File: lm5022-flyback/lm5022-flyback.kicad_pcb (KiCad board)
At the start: 2 copper layers, 80 x 80 mm, 55 parts, among them Q1 EPC2302, SW1 SW_Nidec_CAS-120A1, T1 Arthur, U1 LM5022MM, U2 TLVH431BQDCKT, U3 LTV-817-C

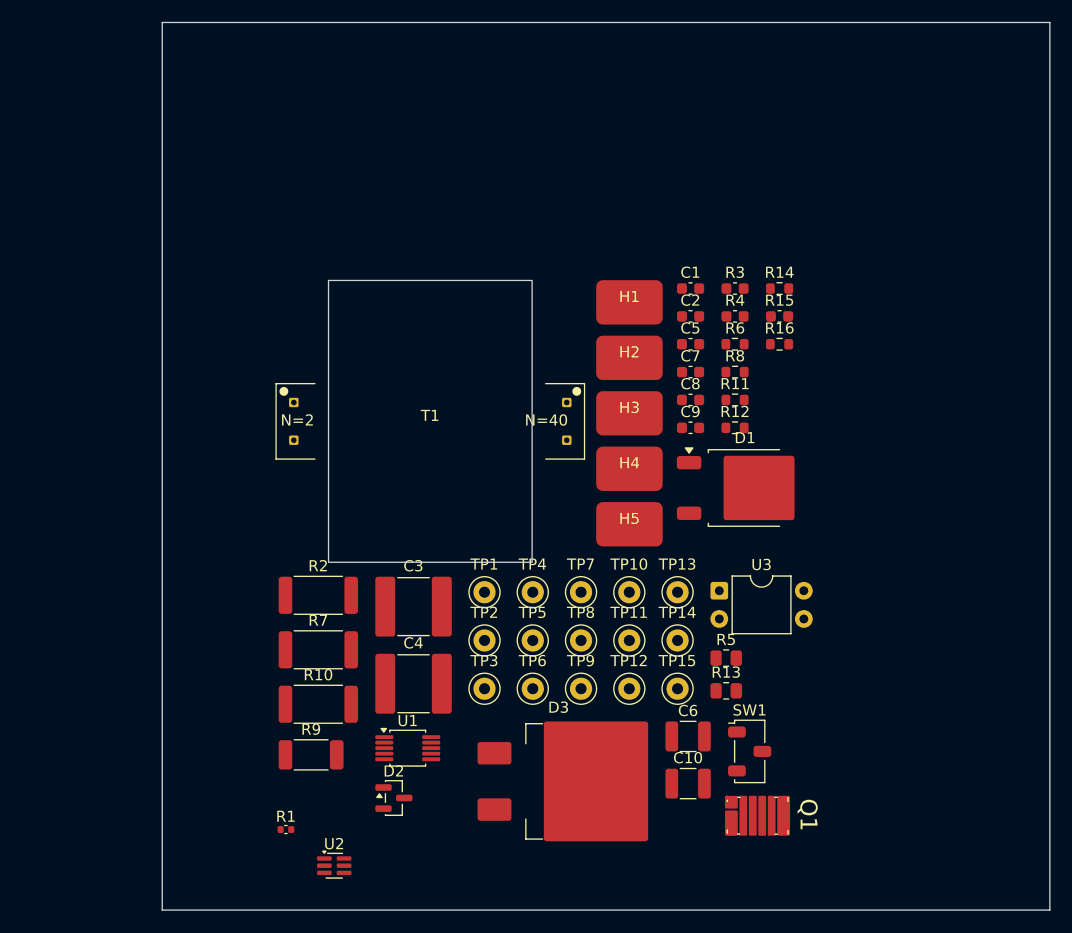
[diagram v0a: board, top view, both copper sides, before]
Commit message: layout work
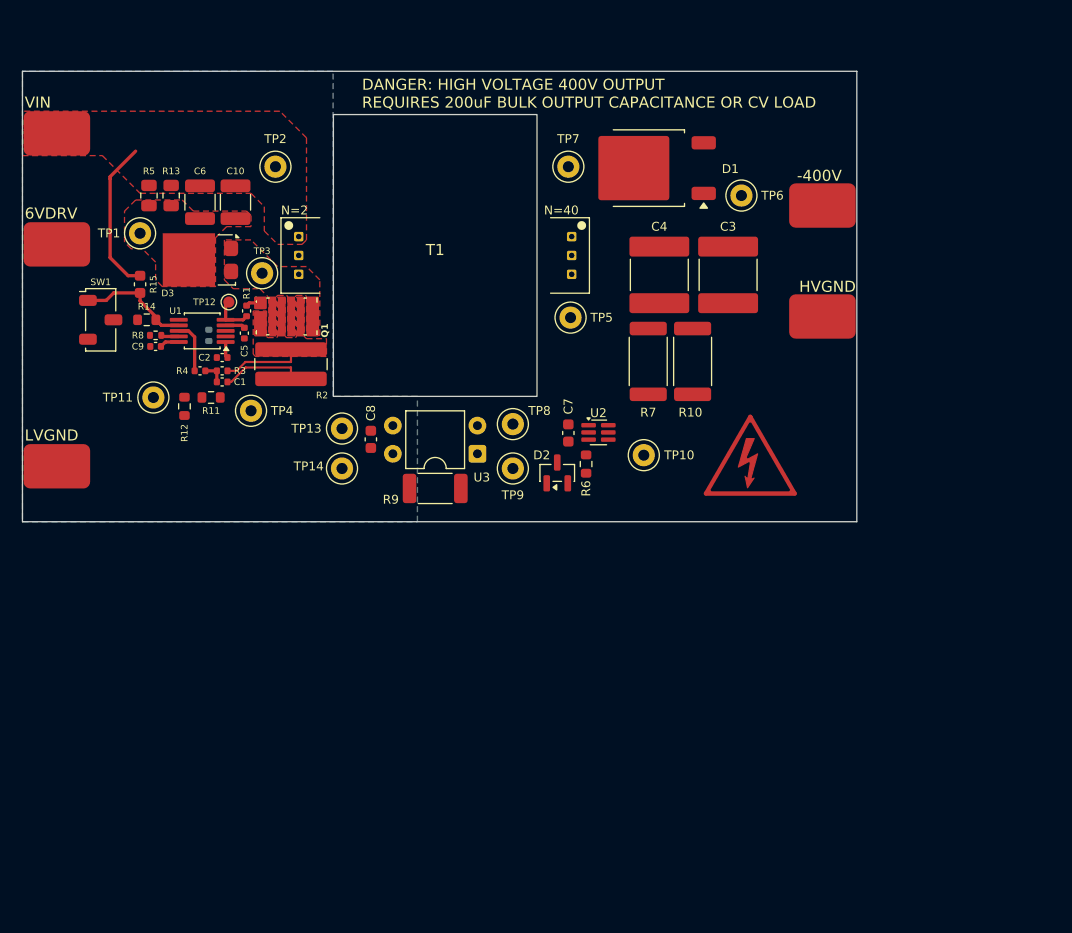
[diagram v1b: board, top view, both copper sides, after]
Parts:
- removed TP15: 5004, TestPoint:TestPoint_Keystone_5000-5004_Miniature
- added REF**: Symbol_HighVoltage_Triangle_8x7mm_Copper, Symbol:Symbol_HighVoltage_Triangle_8x7mm_Copper, F.Cu at (123.0, 104.0)
- C1, C2, C5, C9, R3, R4: footprint Capacitor_SMD:C_0603_1608Metric -> Capacitor_SMD:C_0402_1005Metric
- C8: value 100pF DNP -> 100pF
- D3: value V40D103C-M3/I -> PPH10100; footprint TO_SOT_SMD_Custom:TO-263-2_Diode -> Package_TO_SOT_SMD:TO-277A
- R16: footprint Resistor_SMD:R_0603_1608Metric -> Resistor_SMD:R_0402_1005Metric; moved to B.Cu
- R2: footprint Resistor_SMD:R_2512_6332Metric -> Resistor_SMD:R_1225_3264Metric
- R8: footprint Resistor_SMD:R_0603_1608Metric -> Resistor_SMD:R_0402_1005Metric
- TP12: value 5004 -> ~; footprint TestPoint:TestPoint_Keystone_5000-5004_Miniature -> TestPoint:TestPoint_Pad_D1.0mm
- moved SW1 70.2 mm to (64.5, 91.8)
- moved R13 67.0 mm to (70.8, 80.6), turned to -90 degrees
- moved R5 66.7 mm to (68.8, 80.6), turned to -90 degrees
- moved C10 66.4 mm to (76.6, 81.2), turned to -90 degrees
- moved C6 65.2 mm to (73.4, 81.2), turned to -90 degrees
- moved Q1 61.9 mm to (81.2, 91.5)
- moved D3 58.1 mm to (73.4, 86.4), turned to -90 degrees
- moved R15 57.7 mm to (68.0, 88.6), turned to -90 degrees
- moved H3 57.4 mm to (60.5, 75.0)
- moved H5 57.4 mm to (60.5, 85.0)
- moved R14 57.1 mm to (68.6, 91.8), turned to 180 degrees
- moved R8 52.3 mm to (69.4, 93.2), turned to 180 degrees
- moved H4 51.6 mm to (60.5, 105.0)
- moved R16 51.4 mm to (74.2, 93.2), turned to -90 degrees
- moved TP12 50.2 mm to (76.0, 90.2)
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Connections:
- net Net-(Q1-S-Pad2) renamed /VS
- C10 pad 2: Net-(D3-K) -> /VSN
- C6 pad 2: Net-(D3-K) -> /VSN
- D3 pad 1: Net-(D3-K) -> /VD
- D3 pad 2: Net-(D3-A) -> /VD
- Q1 pad 3: Net-(D3-A) -> /VD
- Q1 pad 5: Net-(D3-A) -> /VD
- Q1 pad 7: Net-(D3-A) -> /VD
- R13 pad 2: Net-(D3-K) -> /VSN
- R5 pad 2: Net-(D3-K) -> /VSN
- T1 pad 2: Net-(D3-A) -> /VD
- TP1 pad 1: Net-(D3-K) -> /VSN
- TP3 pad 1: Net-(D3-A) -> /VD
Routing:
- net +BATT: track 0.00 -> 13.9 mm
- net Net-(SW1-C): track 0.00 -> 10.3 mm
- net GND: track 0.00 -> 7.28 mm
- net /VS: track 0.00 -> 7.18 mm
- net Net-(U1-CS): track 0.00 -> 4.71 mm
- net Net-(U1-OUT): track 0.00 -> 3.74 mm
- net Net-(C1-Pad1): track 0.00 -> 2.04 mm
- net Net-(U1-VCC): track 0.00 -> 1.78 mm
- net Net-(U1-SS): track 0.00 -> 1.77 mm
- net Net-(U1-RT): track 0.00 -> 1.62 mm
- net +6V: track 0.00 -> 1.47 mm
- net Net-(Q1-G): track 0.00 -> 1.35 mm
- added copper zone on F.Cu, net +BATT
- added copper zone on F.Cu, net /VD
- added copper zone on F.Cu, net /VS
- added copper zone on F.Cu, net /VSN
- added copper zone on B.Cu, net GND
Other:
- board size 80 x 80 mm -> 75.2 x 40.6 mm
- board text added: "-400V"
- board text added: "6VDRV"
- board text added: "DANGER: HIGH VOLTAGE 400V OUTPUT REQUIRES 200uF BULK OUTPUT CAPACITANCE OR CV LOAD"
- board text added: "HVGND"
- board text added: "LVGND"
- board text added: "VIN"
